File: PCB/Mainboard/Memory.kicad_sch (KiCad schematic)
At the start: 19 parts, among them J15 RAM Module, U28 M5M4V16160, U33 M5M4V16160

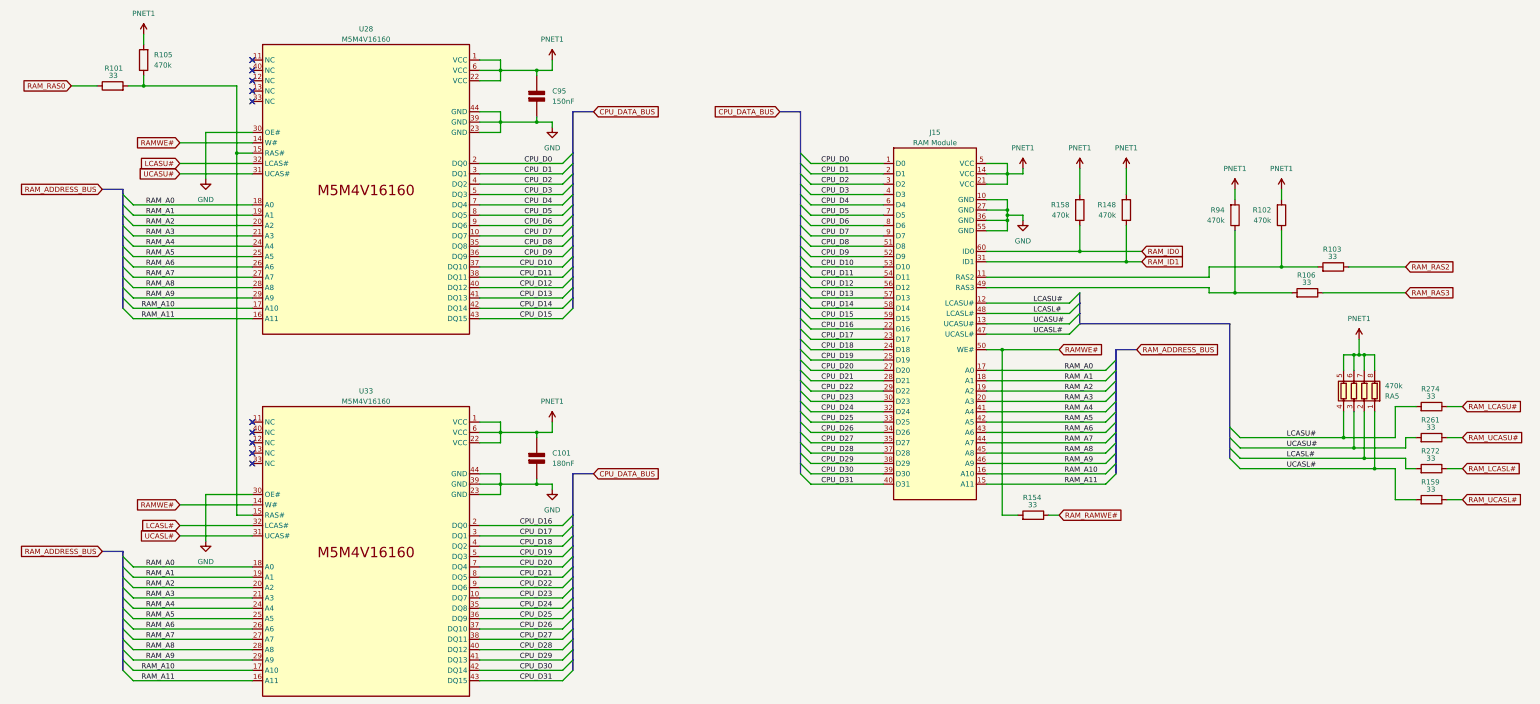
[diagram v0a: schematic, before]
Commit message: Add files via upload
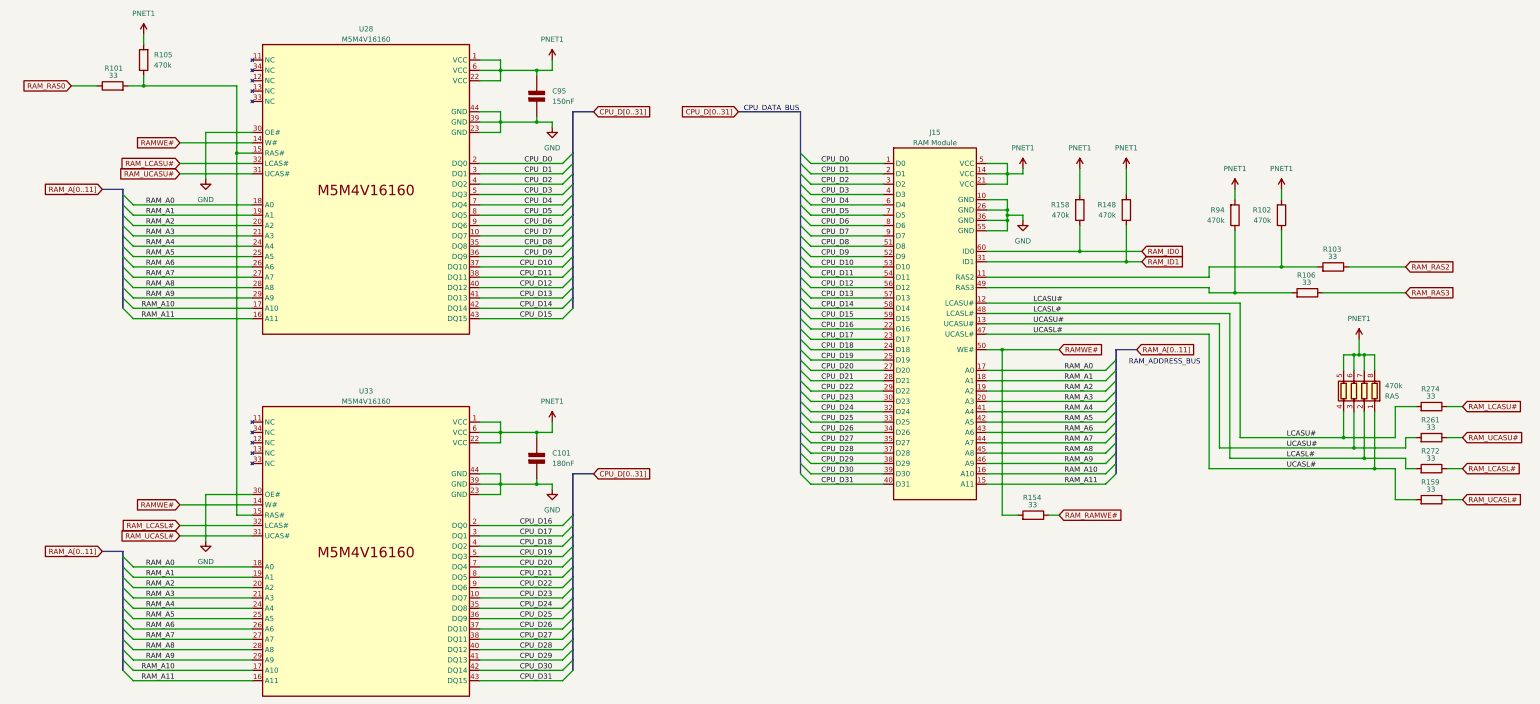
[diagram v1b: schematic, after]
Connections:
- net GND: now also J15.26 (GND); no longer J15.27 (GND)
- net LCASL#: no longer U33.32 (LCAS#)
- net LCASU#: no longer U28.32 (LCAS#)
- net RAM_LCASL#: now also U33.32 (LCAS#)
- net RAM_LCASU#: now also U28.32 (LCAS#)
- net RAM_UCASL#: now also U33.31 (UCAS#)
- net RAM_UCASU#: now also U28.31 (UCAS#)
- net UCASL#: no longer U33.31 (UCAS#)
- net UCASU#: no longer U28.31 (UCAS#)
- no-connect marks 10 -> 0
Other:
- note added: "CPU_DATA_BUS"
- note added: "RAM_ADDRESS_BUS"
